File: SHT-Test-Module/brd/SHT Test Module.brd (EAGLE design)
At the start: 38.1 x 38.1 mm, 13 parts

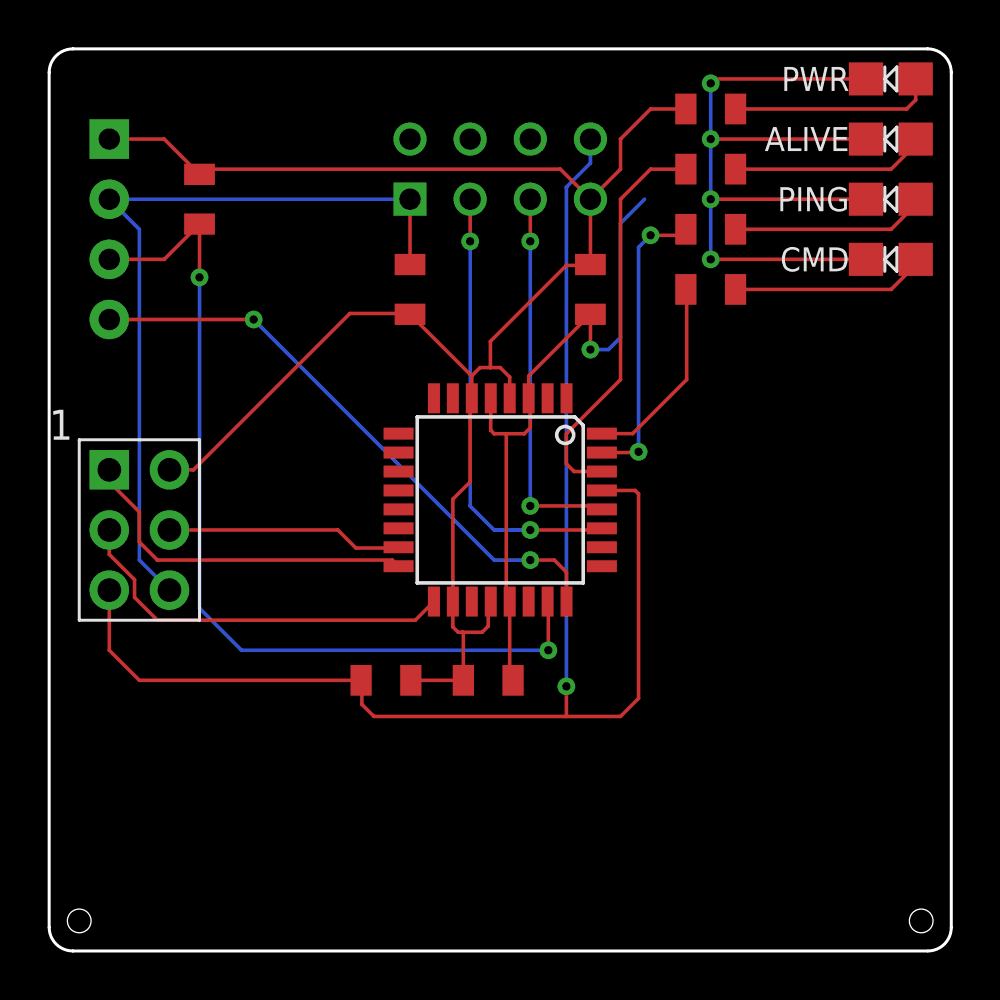
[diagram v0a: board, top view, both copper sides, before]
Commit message: Added SHT board files
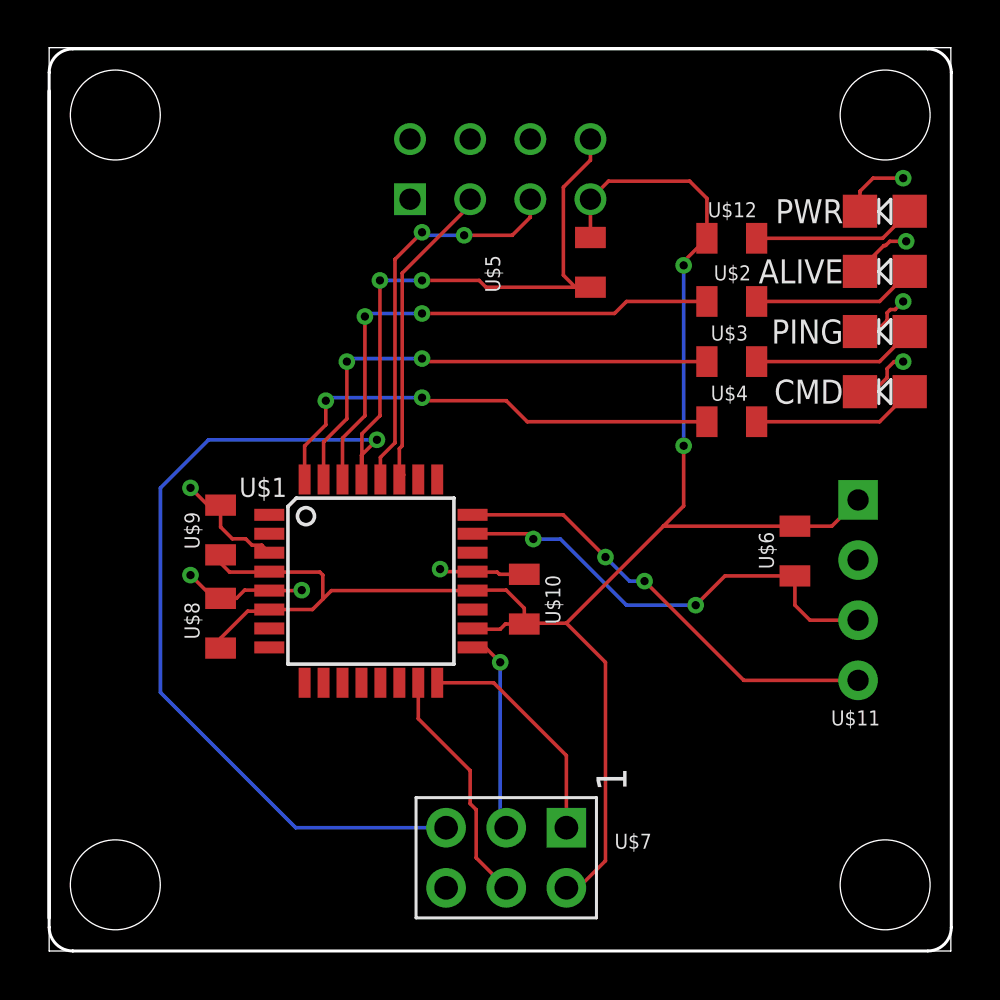
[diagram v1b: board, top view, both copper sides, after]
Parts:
- moved U$11 35.1 mm to (34.2, 15.2)
- moved U$6 29.2 mm to (31.5, 16.9)
- moved U$7 24.5 mm to (21.8, 5.21), turned to 270 degrees
- moved U$8 21.0 mm to (7.24, 13.8), turned to 270 degrees
- moved U$5 19.7 mm to (22.9, 29.1), turned to 90 degrees
- moved U$9 12.9 mm to (7.24, 17.8)
- moved U$1 6.45 mm to (13.6, 15.6), turned to 0 degrees
- moved U$2 5.66 mm to (28.8, 27.4)
- moved U$3 5.66 mm to (28.8, 24.9)
- moved U$4 5.66 mm to (28.8, 22.4)
- moved U$12 5.53 mm to (28.8, 30.1)
- moved U$10 3.75 mm to (20.1, 14.9), turned to 270 degrees
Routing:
- net GND: track 95.7 -> 24.7 mm, vias 5 -> 8
- net DATA: track 38.2 -> 19.5 mm
- net CMD: track 8.35 -> 20.3 mm, vias 0 -> 2
- net PING: track 12.5 -> 20.7 mm
- net SCK: track 16.7 -> 8.52 mm, vias 0 -> 1
- net CLK: track 25.0 -> 19.2 mm
- net SDA: track 19.0 -> 13.4 mm, vias 2 -> 0
- net MISO: track 14.9 -> 9.78 mm
- net ALIVE: track 17.0 -> 22.0 mm, vias 0 -> 2
- net RESET: track 62.0 -> 59.8 mm, vias 1 -> 3
- net N$12: track 8.65 -> 6.94 mm
- net N$15: track 8.27 -> 6.99 mm
- net N$14: track 8.27 -> 6.99 mm
- net N$13: track 8.27 -> 6.99 mm
- net SCL: track 16.0 -> 16.9 mm
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- added copper zone on layer 16, net GND
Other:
- board size 38.1 x 38.1 mm -> 38.1 x 38.2 mm
